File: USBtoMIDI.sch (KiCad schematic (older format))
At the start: 70 parts, among them J1 Conn_01x03, J2 Conn_01x03, J3 Conn_01x03, J7 Conn_02x04_Odd_Even, J8 Conn_01x05, J9 Conn_01x09, Q1 2N2219, Q2 2N2219, Q3 2N2219, Q4 2N2219, Q5 2N2219, SW1 SW_DIP_x04, U1 PIC24FJ64GB002, U2 24LC02, U3 AMS1117-3.3, U4 74HC14, U5 74HC14, U6 6N139, U7 4081, Y1 16MHz

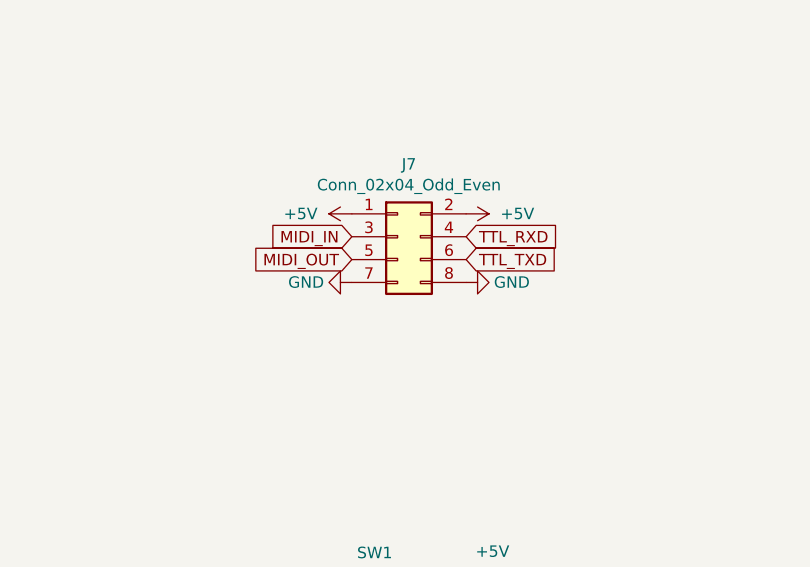
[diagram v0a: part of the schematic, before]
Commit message: update config ports
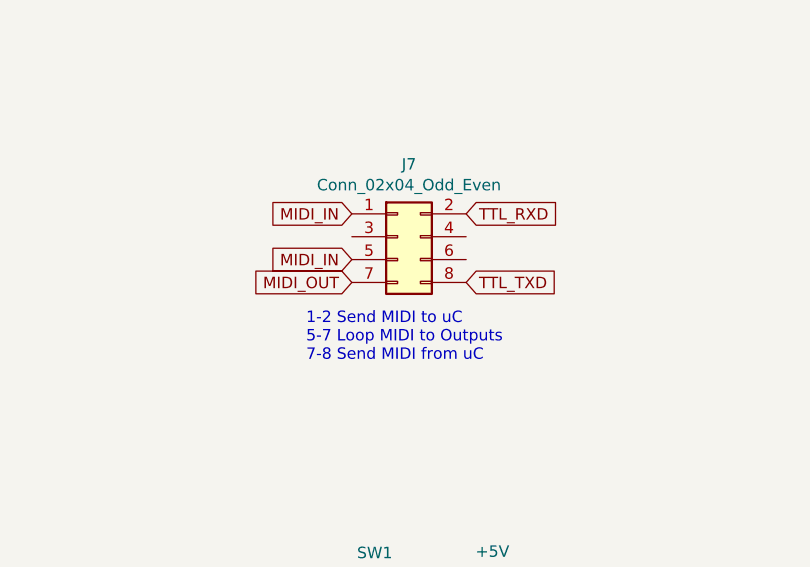
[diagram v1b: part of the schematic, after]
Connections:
- net +5V: no longer J7.1 (Pin_1), J7.2 (Pin_2)
- net GND: no longer J7.7 (Pin_7), J7.8 (Pin_8)
- net MIDI_IN: now also J7.1 (Pin_1), J7.5 (Pin_5); no longer J7.3 (Pin_3)
- net MIDI_OUT: now also J7.7 (Pin_7); no longer J7.5 (Pin_5)
- net TTL_RXD: now also J7.2 (Pin_2); no longer J7.4 (Pin_4)
- net TTL_TXD: now also J7.8 (Pin_8); no longer J7.6 (Pin_6)
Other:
- note added: "1-2 Send MIDI to uC\n5-7 Loop MIDI to Outputs\n7-8 Send MIDI from uC"
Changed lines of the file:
@@
 	1    0    0    -1
 $EndComp
-Text GLabel 8100 5850 0    50   Input ~ 0
+Text GLabel 8100 5950 0    50   Input ~ 0
 MIDI_IN
-Text GLabel 8100 5950 0    50   Input ~ 0
+Text GLabel 8100 6050 0    50   Input ~ 0
 MIDI_OUT
-$Comp
-L power:GND #PWR0146
-U 1 1 601A1DE5
-P 8100 6050
-F 0 "#PWR0146" H 8100 5800 50  0001 C CNN
-F 1 "GND" V 8100 5850 50  0000 C CNN
-F 2 "" H 8100 6050 50  0001 C CNN
-F 3 "" H 8100 6050 50  0001 C CNN
-	1    8100 6050
-	0    1    1    0
-$EndComp
-$Comp
-L power:+5V #PWR0147
-U 1 1 601A27C1
-P 8100 5750
-F 0 "#PWR0147" H 8100 5600 50  0001 C CNN
-F 1 "+5V" V 8100 5900 50  0000 L CNN
-F 2 "" H 8100 5750 50  0001 C CNN
-F 3 "" H 8100 5750 50  0001 C CNN
-	1    8100 5750
-	0    -1   -1   0
-$EndComp
 $Comp
 L power:GND #PWR0148
@@
 	1    8300 5850
 	1    0    0    -1
-$EndComp
-Text GLabel 8600 5850 2    50   Input ~ 0
-TTL_RXD
-Text GLabel 8600 5950 2    50   Input ~ 0
-TTL_TXD
-$Comp
-L power:+5V #PWR0149
-U 1 1 601B6FFF
-P 8600 5750
-F 0 "#PWR0149" H 8600 5600 50  0001 C CNN
-F 1 "+5V" V 8600 5900 50  0000 L CNN
-F 2 "" H 8600 5750 50  0001 C CNN
-F 3 "" H 8600 5750 50  0001 C CNN
-	1    8600 5750
-	0    1    1    0
-$EndComp
-$Comp
-L power:GND #PWR0150
-U 1 1 601B7A49
-P 8600 6050
-F 0 "#PWR0150" H 8600 5800 50  0001 C CNN
-F 1 "GND" V 8600 5850 50  0000 C CNN
-F 2 "" H 8600 6050 50  0001 C CNN
-F 3 "" H 8600 6050 50  0001 C CNN
-	1    8600 6050
-	0    -1   -1   0
 $EndComp
 Text GLabel 11350 2650 2    50   Input ~ 0
@@
 Wire Wire Line
 	7800 7500 7900 7500
+Text GLabel 8100 5750 0    50   Input ~ 0
+MIDI_IN
+Text GLabel 8600 5750 2    50   Input ~ 0
+TTL_RXD
+Text GLabel 8600 6050 2    50   Input ~ 0
+TTL_TXD
+Text Notes 7900 6400 0    50   ~ 0
+1-2 Send MIDI to uC\n5-7 Loop MIDI to Outputs\n7-8 Send MIDI from uC
 $EndSCHEMATC
